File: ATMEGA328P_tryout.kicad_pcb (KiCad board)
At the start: 2 copper layers, 115 x 95 mm, 39 parts, among them J1 Conn_01x08, J2 Conn_01x06, J3 Conn_01x06, J4 Conn_01x08, J5 Conn_01x03, J6 Conn_01x03, J7 Conn_01x02, J8 USB_B_Mini, SW1 SW_Push, U1 ATMEGA328P, U2 AMS1117-3.3, U3 AMS1117-5.0, U4 CP2104, Y1 O16M

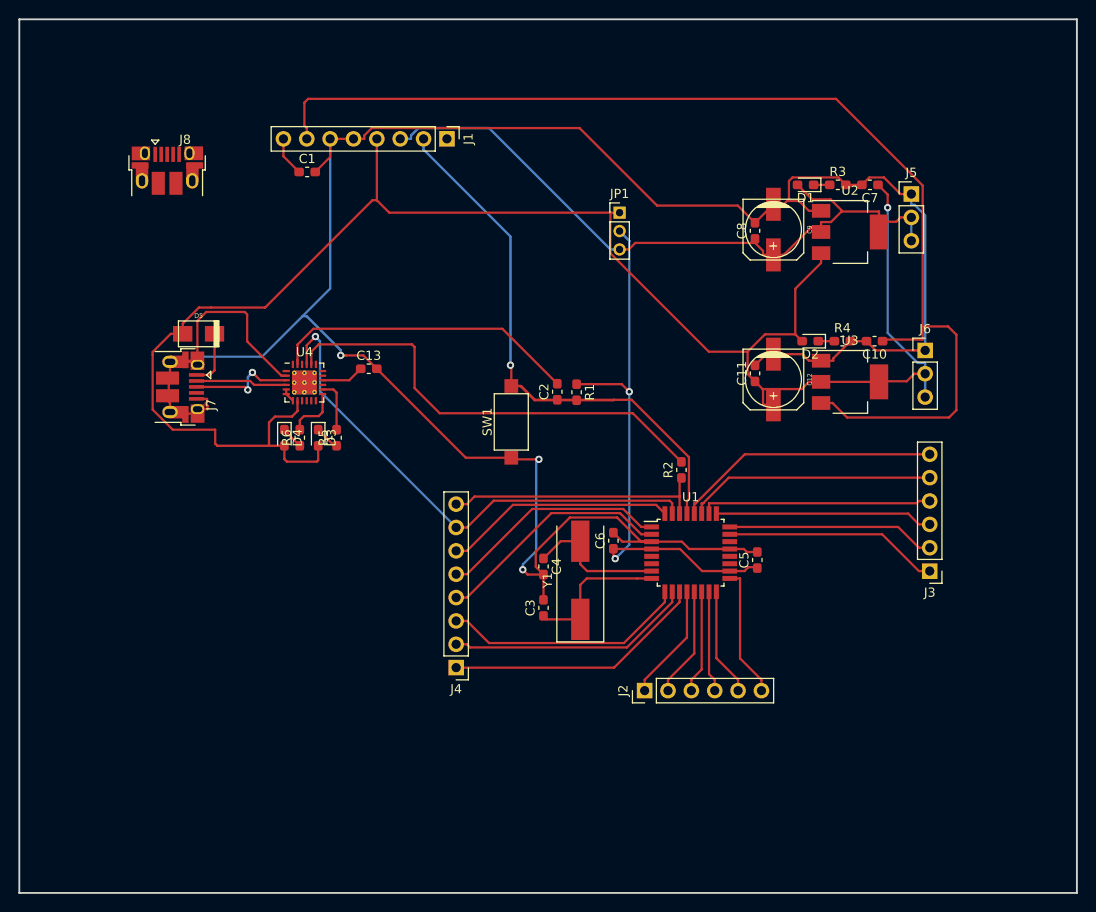
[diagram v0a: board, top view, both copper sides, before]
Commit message: update,
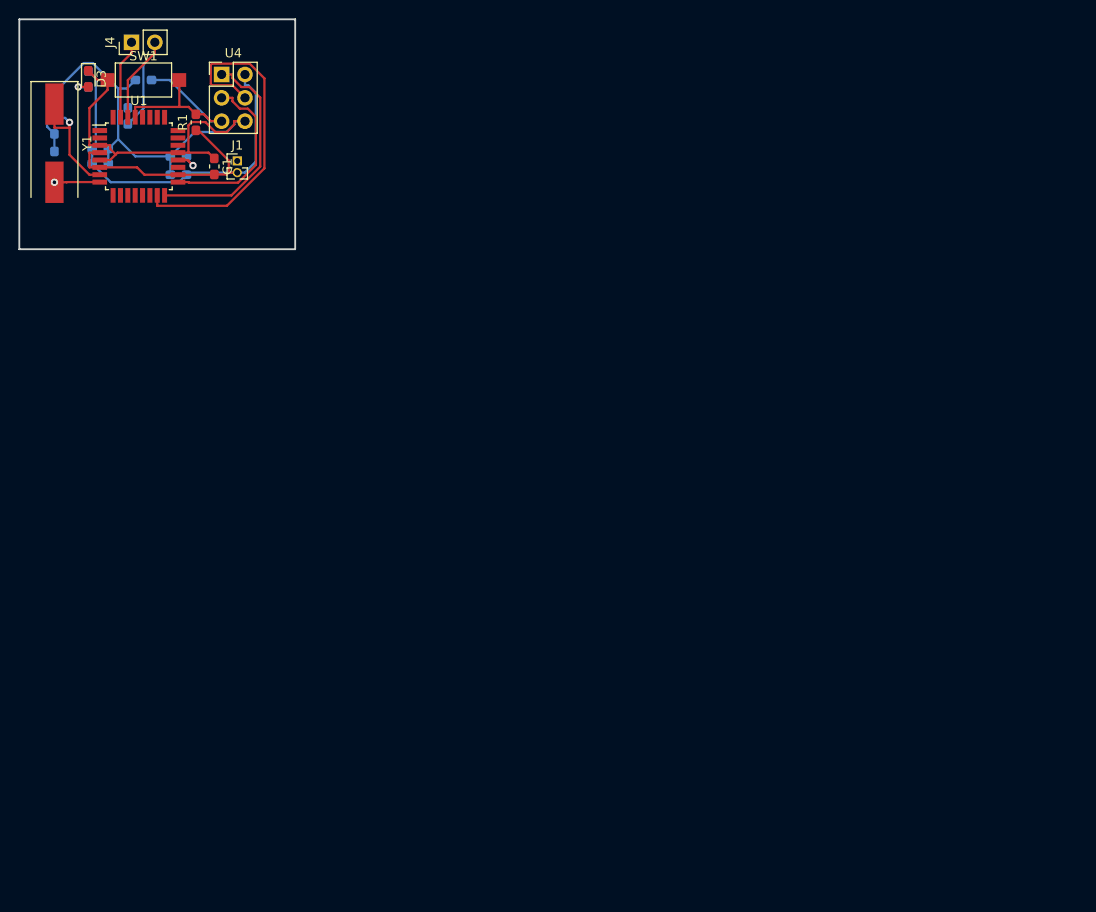
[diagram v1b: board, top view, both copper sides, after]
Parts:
- removed C10, C11, C7, C8: C104,0603, Capacitor_SMD:C_0603_1608Metric_Pad1.05x0.95mm_HandSolder
- removed C12, C9: CP47uf,50V, w_smd_cap:c_elec_6.3x7.7
- removed D1, D2: LED_GREEN,0603, LED_SMD:LED_0603_1608Metric_Pad1.05x0.95mm_HandSolder
- removed D4: LED_ORANGE,0603, LED_SMD:LED_0603_1608Metric_Pad1.05x0.95mm_HandSolder
- removed D5: SD_1N4001_M1, w_smd_diode:do214ac
- removed J2, J3: Conn_01x06, Connector_PinHeader_2.54mm:PinHeader_1x06_P2.54mm_Vertical
- removed J5, J6: Conn_01x03, Connector_PinHeader_2.54mm:PinHeader_1x03_P2.54mm_Vertical
- removed J7: Conn_01x02, Connector_USB:USB_Micro-B_Amphenol_10103594-0001LF_Horizontal
- removed J8: USB_B_Mini, Connector_USB:USB_Micro-B_Amphenol_10103594-0001LF_Horizontal
- removed JP1: Jumper_3_Bridged12, Connector_PinHeader_2.00mm:PinHeader_1x03_P2.00mm_Vertical
- removed R3, R4, R6: R102,0603, Resistor_SMD:R_0603_1608Metric_Pad1.05x0.95mm_HandSolder
- removed U2: AMS1117-3.3, Package_TO_SOT_SMD:SOT-223-3_TabPin2
- removed U3: AMS1117-5.0, Package_TO_SOT_SMD:SOT-223-3_TabPin2
- added C14: C105,0603, Capacitor_SMD:C_0603_1608Metric_Pad1.05x0.95mm_HandSolder, B.Cu at (37.3, 41.9)
- C1: value C104,0603 -> C106,0603
- C13: value C106,0603 -> C104,0603; moved to B.Cu
- C2, C3, C4, C5, C6, R2: moved to B.Cu
- D3: value LED_ORANGE,0603 -> LED_GREEN,0603
- J1: value Conn_01x08 -> Conn_01x02; footprint Connector_PinHeader_2.54mm:PinHeader_1x08_P2.54mm_Vertical -> Connector_PinHeader_1.27mm:PinHeader_1x02_P1.27mm_Vertical
- J4: value Conn_01x08 -> Conn_01x02; footprint Connector_PinHeader_2.54mm:PinHeader_1x08_P2.54mm_Vertical -> Connector_PinHeader_2.54mm:PinHeader_1x02_P2.54mm_Vertical
- R5: value R102,0603 -> R103,0603; moved to B.Cu
- U1: value ATMEGA328P -> ATMEGA328P-TQFP
- U4: value CP2104 -> CONN_ARDUINO_ICSP; footprint Package_DFN_QFN:QFN-24-1EP_4x4mm_P0.5mm_EP2.7x2.6mm_ThermalVias -> Connector_PinHeader_2.54mm:PinHeader_2x03_P2.54mm_Vertical
- moved C5 84.3 mm to (28.8, 39.1), turned to 0 degrees
- moved J4 76.6 mm to (32.2, 27.5), turned to 90 degrees
- moved C3 74.7 mm to (23.8, 36.6), turned to 270 degrees
- moved Y1 74.4 mm to (23.8, 38.5), turned to 270 degrees
- moved U1 73.9 mm to (33.0, 39.9)
- moved R2 71.5 mm to (31.8, 35.5), turned to 270 degrees
- moved C6 69.2 mm to (28.8, 40.7), turned to 0 degrees
- moved C4 69.2 mm to (23.8, 40.2), turned to 90 degrees
- moved C2 56.3 mm to (33.5, 31.6), turned to 180 degrees
- moved SW1 54.6 mm to (33.5, 31.6), turned to 0 degrees
- moved R1 50.7 mm to (39.2, 36.2), turned to 90 degrees
- moved R5 47.4 mm to (27.5, 31.5)
- moved D3 46.3 mm to (27.5, 31.5)
- moved U4 34.7 mm to (42.0, 31.0)
- moved C13 31.0 mm to (37.3, 39.9), turned to 180 degrees
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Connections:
- C1 pad 1: Net-(C1-Pad1) -> GND
- C1 pad 2: GND -> VCC
- C2 pad 1: RESET -> /ATMEGA328P/RESET
- C5 pad 1: VCCIO -> VCC
- C6 pad 1: VCCIO -> VCC
- D3 pad 1: Net-(D3-Pad1) -> GND
- D3 pad 2: +5V -> Net-(D3-Pad2)
- J1 pad 1: VBUS -> +5V
- J1 pad 2: RESET -> VCC
- J4 pad 1: Net-(J4-Pad1) -> TXD
- R1 pad 1: VCCIO -> VCC
- R1 pad 2: RESET -> /ATMEGA328P/RESET
- R2 pad 1: Net-(J4-Pad8) -> RXD
- R2 pad 2: RXD -> Net-(J4-Pad2)
- R5 pad 1: Net-(D3-Pad1) -> Net-(D3-Pad2)
- R5 pad 2: Net-(R5-Pad2) -> VCC
- SW1 pad 2: RESET -> /ATMEGA328P/RESET
- U1 pad 1: Net-(J4-Pad5) -> Net-(U1-Pad1)
- U1 pad 10: Net-(J4-Pad2) -> Net-(U1-Pad10)
- U1 pad 11: Net-(J4-Pad1) -> Net-(U1-Pad11)
- U1 pad 15: Net-(J2-Pad4) -> /ATMEGA328P/MOSI
- U1 pad 16: Net-(J2-Pad5) -> /ATMEGA328P/MISO
- U1 pad 17: Net-(J2-Pad6) -> /ATMEGA328P/SCK
- U1 pad 18: VCCIO -> VCC
- U1 pad 19: (no net) -> Net-(U1-Pad19)
- U1 pad 2: Net-(J4-Pad4) -> Net-(U1-Pad2)
- U1 pad 20: AREF -> Net-(C13-Pad1)
- U1 pad 22: (no net) -> Net-(U1-Pad22)
- U1 pad 29: RESET -> /ATMEGA328P/RESET
- U1 pad 30: Net-(J4-Pad8) -> Net-(J4-Pad2)
- U1 pad 32: Net-(J4-Pad6) -> Net-(U1-Pad32)
- U1 pad 4: VCCIO -> VCC
- U1 pad 5: (no net) -> GND
- U1 pad 6: (no net) -> VCC
- U1 pad 7: Net-(C4-Pad1) -> Net-(C3-Pad1)
- U1 pad 8: Net-(C3-Pad1) -> Net-(C4-Pad1)
- U1 pad 9: Net-(J4-Pad3) -> Net-(U1-Pad9)
- U4 pad 1: Net-(U4-Pad1) -> /ATMEGA328P/MISO
- U4 pad 2: GND -> VCC
- U4 pad 3: D_P -> /ATMEGA328P/SCK
- U4 pad 4: D_M -> /ATMEGA328P/MOSI
- U4 pad 5: +3V3 -> /ATMEGA328P/RESET
- U4 pad 6: +3V3 -> GND
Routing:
- net +5V: track 194.8 -> 0.00 mm, vias 1 -> 0
- net GND: track 275.8 -> 83.1 mm, vias 3 -> 0
- net VIN: track 124.5 -> 0.00 mm
- net +3V3: track 78.6 -> 0.00 mm
- net RESET: track 71.4 -> 0.00 mm, vias 1 -> 0
- net VCC: track 0.00 -> 65.8 mm
- net VCCIO: track 60.8 -> 0.00 mm, vias 2 -> 0
- net RXD: track 49.9 -> 0.00 mm
- net TXD: track 56.5 -> 8.65 mm, vias 1 -> 0
- net /ATMEGA328P/MOSI: track 0.00 -> 37.2 mm
- net DTR: track 33.6 -> 0.00 mm
- net Net-(U1-Pad28): track 28.9 -> 0.00 mm
- net Net-(J4-Pad8): track 28.6 -> 0.00 mm
- net Net-(J4-Pad1): track 28.4 -> 0.00 mm
- net Net-(U1-Pad27): track 27.1 -> 0.00 mm
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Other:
- board size 115 x 95 mm -> 30 x 25 mm
